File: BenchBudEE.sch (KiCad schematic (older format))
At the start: 0 parts

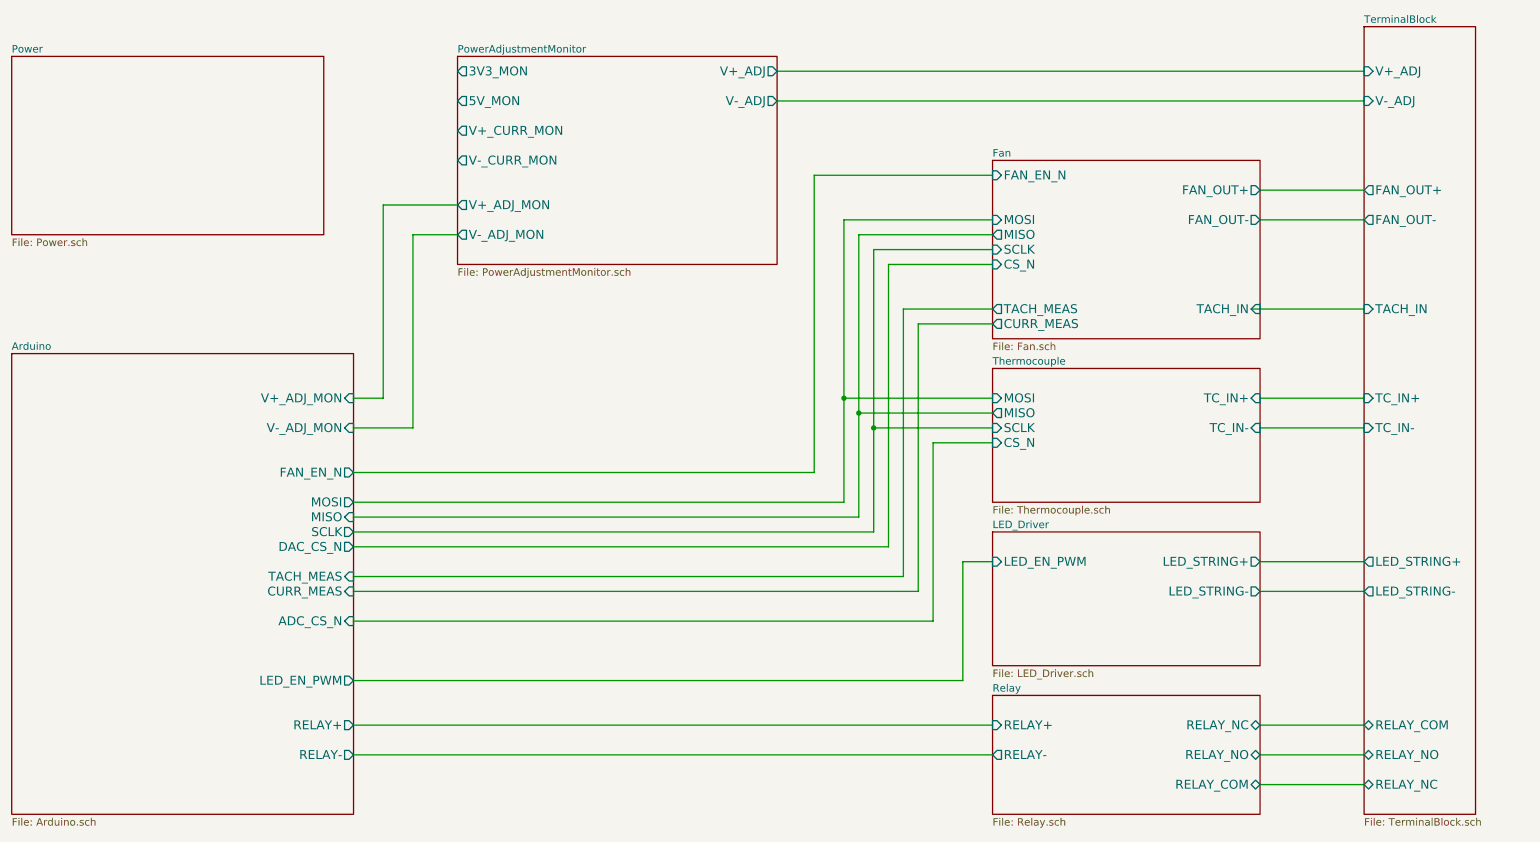
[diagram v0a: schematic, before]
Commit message: Some cleanup/fixes on the top-level
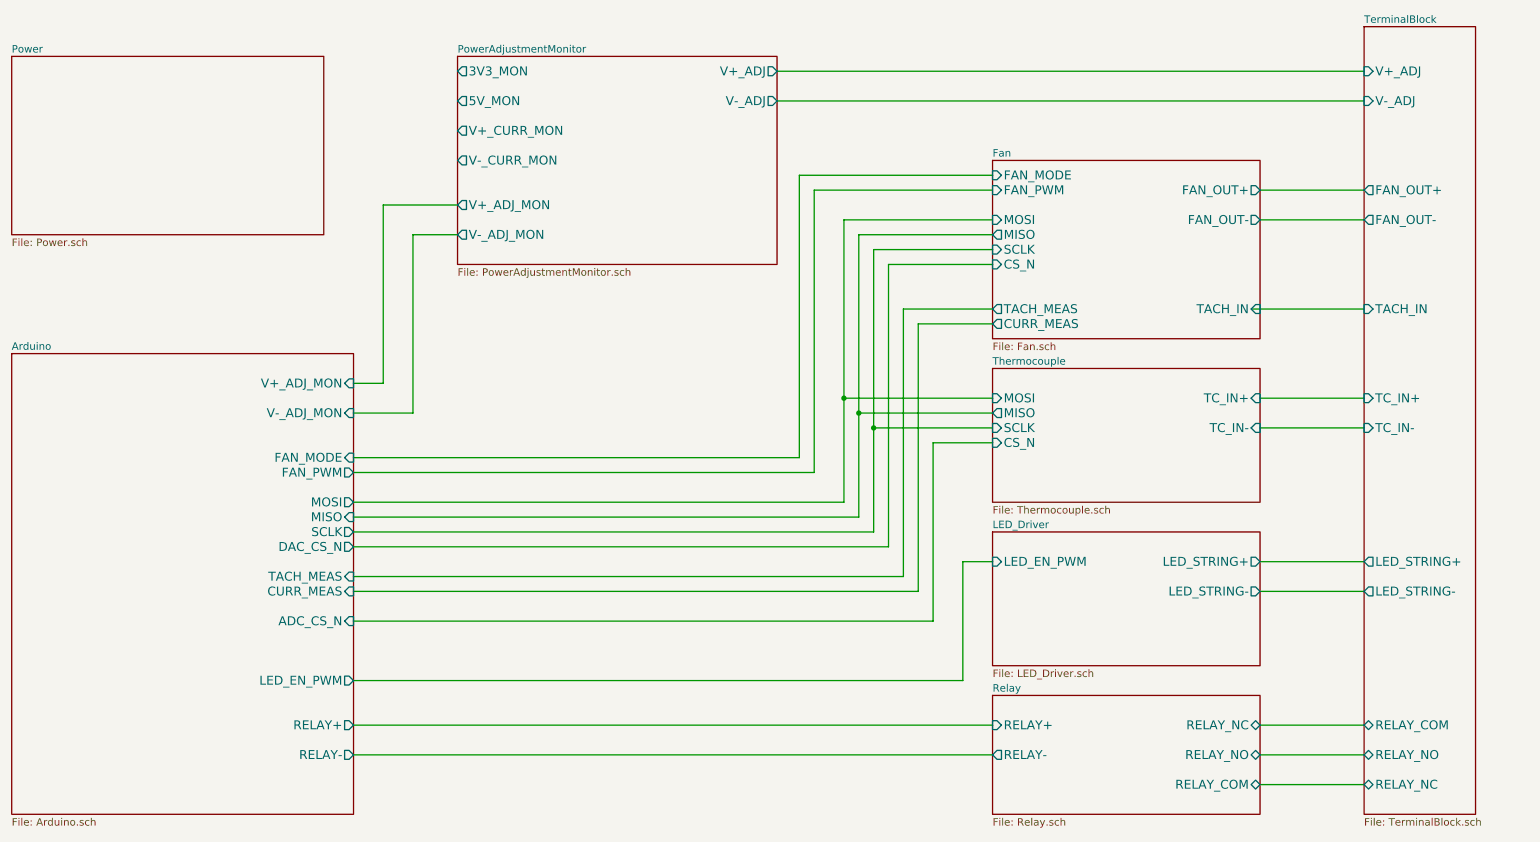
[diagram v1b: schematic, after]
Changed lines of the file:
@@
 	10000 5900 9300 5900
 Wire Wire Line
-	3200 3300 3400 3300
+	3200 3200 3400 3200
 Wire Wire Line
-	3400 3300 3400 2000
+	3400 3200 3400 2000
 Wire Wire Line
 	3400 2000 3900 2000
 Wire Wire Line
-	3200 3500 3600 3500
+	3200 3400 3600 3400
 Wire Wire Line
-	3600 3500 3600 2200
+	3600 3400 3600 2200
 Wire Wire Line
 	3600 2200 3900 2200
@@
 	3200 3800 6300 3800
 Wire Wire Line
-	6300 3800 6300 1800
+	6300 3800 6300 1900
 Wire Wire Line
-	6300 1800 7500 1800
+	6300 1900 7500 1900
 Wire Wire Line
 	6500 4000 3200 4000
 Wire Wire Line
-	6500 2100 6500 4000
+	6500 2100 6500 3300
+Wire Wire Line
+	6500 3300 6500 4000
 Wire Wire Line
 	6500 2100 7500 2100
@@
 	6600 4100 3200 4100
 Wire Wire Line
-	6600 2200 6600 4100
+	6600 2200 6600 3400
+Wire Wire Line
+	6600 3400 6600 4100
 Wire Wire Line
 	6600 2200 7500 2200
@@
 	6700 4200 3200 4200
 Wire Wire Line
-	6700 2300 6700 4200
+	6700 2300 6700 3500
+Wire Wire Line
+	6700 3500 6700 4200
 Wire Wire Line
 	6700 2300 7500 2300
@@
 F7 "TACH_IN" I R 9300 2700 60
 F8 "TACH_MEAS" O L 7500 2700 60
-F9 "FAN_EN_N" I L 7500 1800 60
-F10 "CURR_MEAS" O L 7500 2800 60
-F11 "FAN_OUT-" O R 9300 2100 60
+F9 "CURR_MEAS" O L 7500 2800 60
+F10 "FAN_OUT-" O R 9300 2100 60
+F11 "FAN_PWM" I L 7500 1900 60
+F12 "FAN_MODE" I L 7500 1800 60
 $EndSheet
 $Sheet
@@
 F4 "TACH_MEAS" I R 3200 4500 60
 F5 "SCLK" O R 3200 4200 60
-F6 "FAN_EN_N" O R 3200 3800 60
-F7 "CURR_MEAS" I R 3200 4600 60
-F8 "RELAY+" O R 3200 5500 60
-F9 "RELAY-" O R 3200 5700 60
-F10 "V+_ADJ_MON" I R 3200 3300 60
-F11 "V-_ADJ_MON" I R 3200 3500 60
-F12 "LED_EN_PWM" O R 3200 5200 60
-F13 "DAC_CS_N" O R 3200 4300 60
-F14 "ADC_CS_N" I R 3200 4800 60
+F6 "CURR_MEAS" I R 3200 4600 60
+F7 "RELAY+" O R 3200 5500 60
+F8 "RELAY-" O R 3200 5700 60
+F9 "V+_ADJ_MON" I R 3200 3200 60
+F10 "V-_ADJ_MON" I R 3200 3400 60
+F11 "LED_EN_PWM" O R 3200 5200 60
+F12 "DAC_CS_N" O R 3200 4300 60
+F13 "ADC_CS_N" I R 3200 4800 60
+F14 "FAN_PWM" O R 3200 3800 60
+F15 "FAN_MODE" I R 3200 3700 60
 $EndSheet
 Wire Wire Line
@@
 Wire Wire Line
 	7500 5700 3200 5700
+Wire Wire Line
+	7500 1800 6200 1800
+Wire Wire Line
+	6200 1800 6200 3700
+Wire Wire Line
+	6200 3700 3200 3700
 $EndSCHEMATC
